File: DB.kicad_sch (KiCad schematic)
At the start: 20 parts

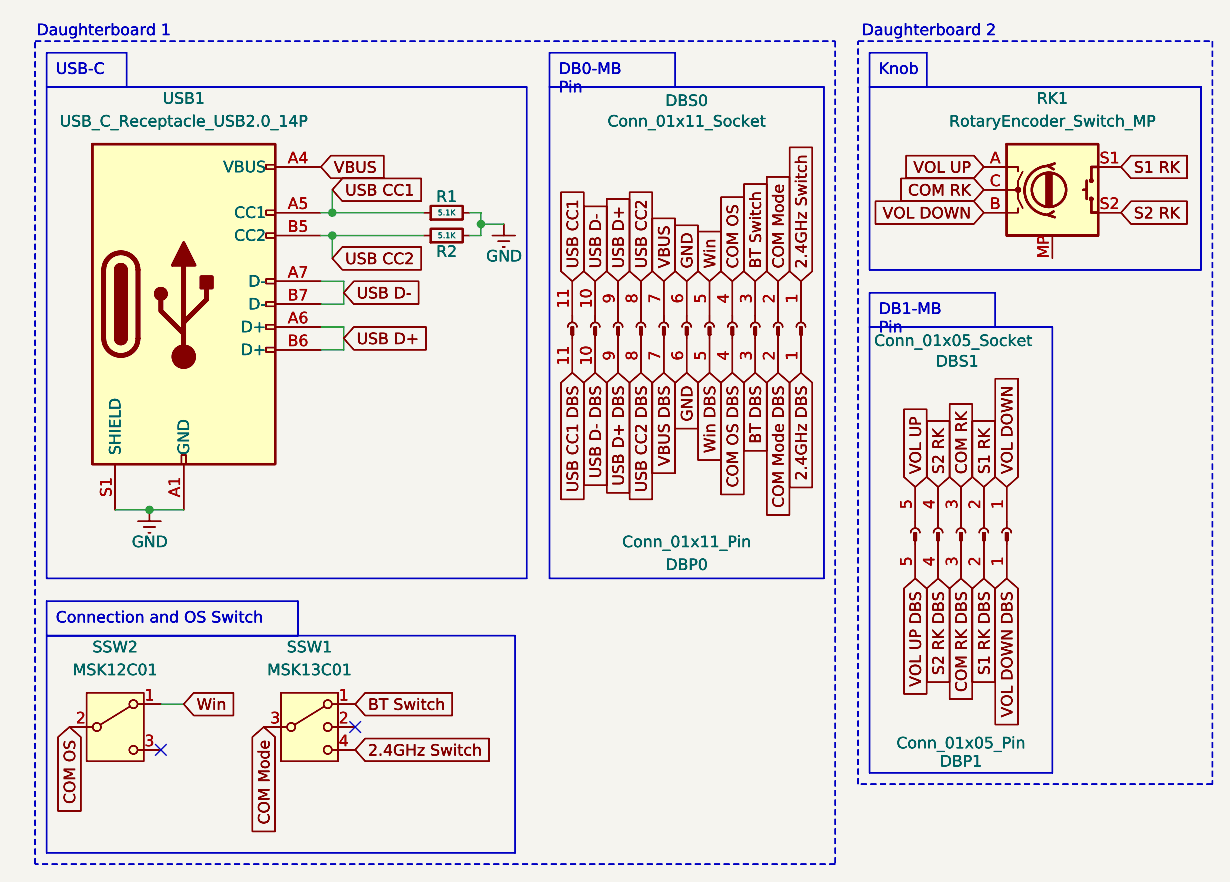
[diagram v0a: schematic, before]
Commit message: Second Commit
new wiring and label
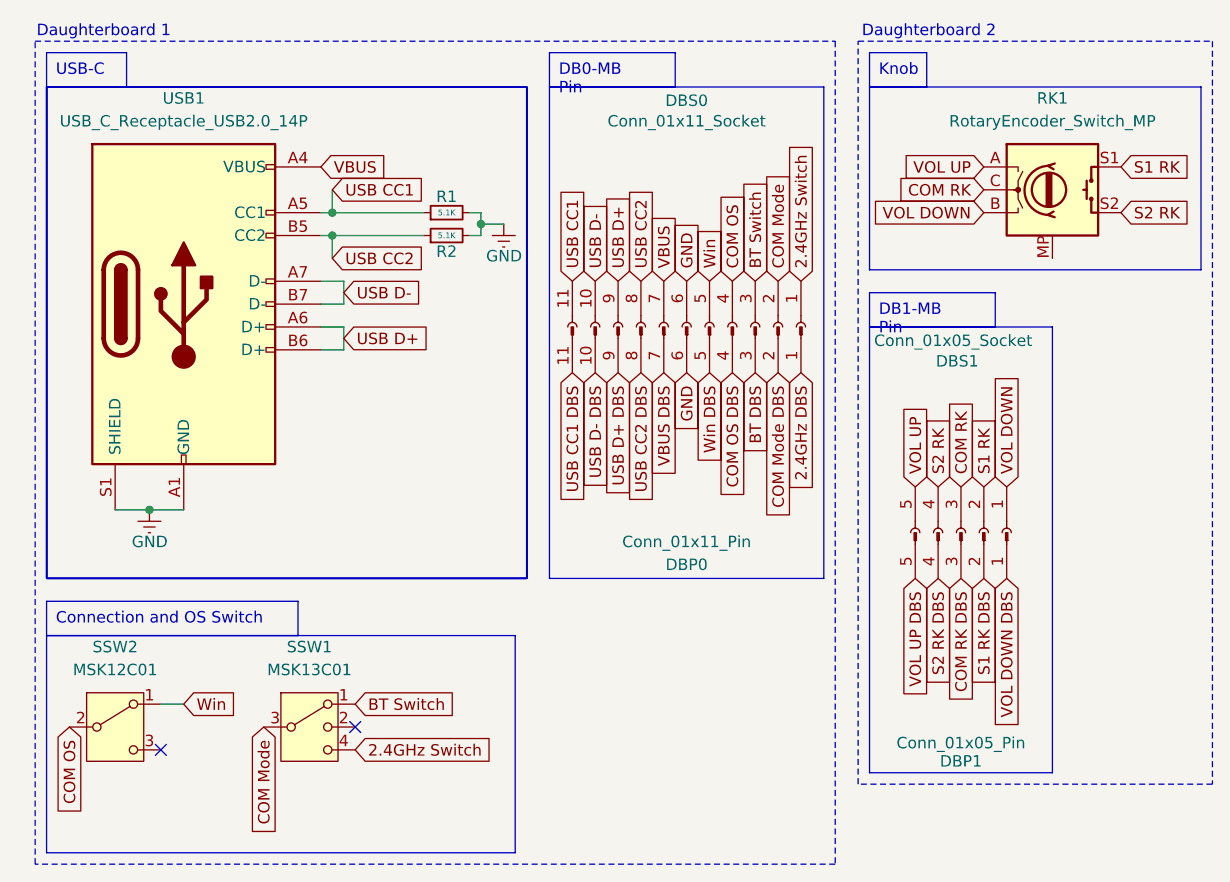
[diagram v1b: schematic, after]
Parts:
- removed DBP0: Conn_01x11_Pin, symbol Connector:Conn_01x11_Pin
- removed DBP1 (x2): Conn_01x05_Pin, symbol Connector:Conn_01x05_Pin
- removed DBS0: Conn_01x11_Socket, Connector_Molex:Molex_PicoBlade_53261-1171_1x11-1MP_P1.25mm_Horizontal, symbol Connector:Conn_01x11_Socket
- removed DBS1: Conn_01x05_Socket, Connector_Molex:Molex_PicoBlade_53261-0571_1x05-1MP_P1.25mm_Horizontal, symbol Connector:Conn_01x05_Socket
- removed R1, R2 (x2): 5.1K, ScottoKeebs_Components:Resistor_0402, symbol Device:R_Small
- removed RK1: RotaryEncoder_Switch_MP, Rotary_Encoder:RotaryEncoder_Alps_EC11E-Switch_Vertical_H20mm, symbol Device:RotaryEncoder_Switch_MP
- removed SSW1 (x2): MSK13C01, Button_Switch_SMD:SW_SP3T_PCM13, symbol Switch:SW_SP3T
- removed SSW2 (x2): MSK12C01, Button_Switch_SMD:SW_SPDT_PCM12, symbol Switch:SW_SPDT
- removed USB1 (x2): USB_C_Receptacle_USB2.0_14P, ScottoKeebs_Components:USB_C_HRO_TYPE-C-31-M-12, symbol Connector:USB_C_Receptacle_USB2.0_14P
- added DBP1: Conn_01x05_Pin, symbol Connector:Conn_01x05_Pin
- added R2: 5.1K, ScottoKeebs_Components:Resistor_0402, symbol Device:R_Small
- added SSW1: MSK13C01, Button_Switch_SMD:SW_SP3T_PCM13, symbol Switch:SW_SP3T
- added SSW2: MSK12C01, Button_Switch_SMD:SW_SPDT_PCM12, symbol Switch:SW_SPDT
- added USB1: USB_C_Receptacle_USB2.0_14P, ScottoKeebs_Components:USB_C_HRO_TYPE-C-31-M-12, symbol Connector:USB_C_Receptacle_USB2.0_14P
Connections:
- net 2.4GHz Switch: now also SSW1.4
- net BT Switch: now also SSW1.1
- net COM Mode: now also SSW1.3
- net COM OS: now also SSW2.2 (B)
- net COM RK DBS: now also DBP1.3 (Pin_3)
- net GND: now also R2.2, USB1.A1 (GND), USB1.A12 (GND), USB1.B1 (GND), USB1.B12 (GND), USB1.S1 (SHIELD)
- net S1 RK DBS: now also DBP1.2 (Pin_2)
- net S2 RK DBS: now also DBP1.4 (Pin_4)
- net USB CC1: now also USB1.A5 (CC1)
- net USB CC2: now also R2.1, USB1.B5 (CC2)
- net USB D+: now also USB1.A6 (D+), USB1.B6 (D+)
- net USB D-: now also USB1.A7 (D-), USB1.B7 (D-)
- net VBUS: now also USB1.A4 (VBUS), USB1.A9 (VBUS), USB1.B4 (VBUS), USB1.B9 (VBUS)
- net VOL DOWN DBS: now also DBP1.1 (Pin_1)
- net VOL UP DBS: now also DBP1.5 (Pin_5)
- net Win: now also SSW2.1 (A)

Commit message: Third Commit
Kinda add some little changes but still confused on how using the nPM1300
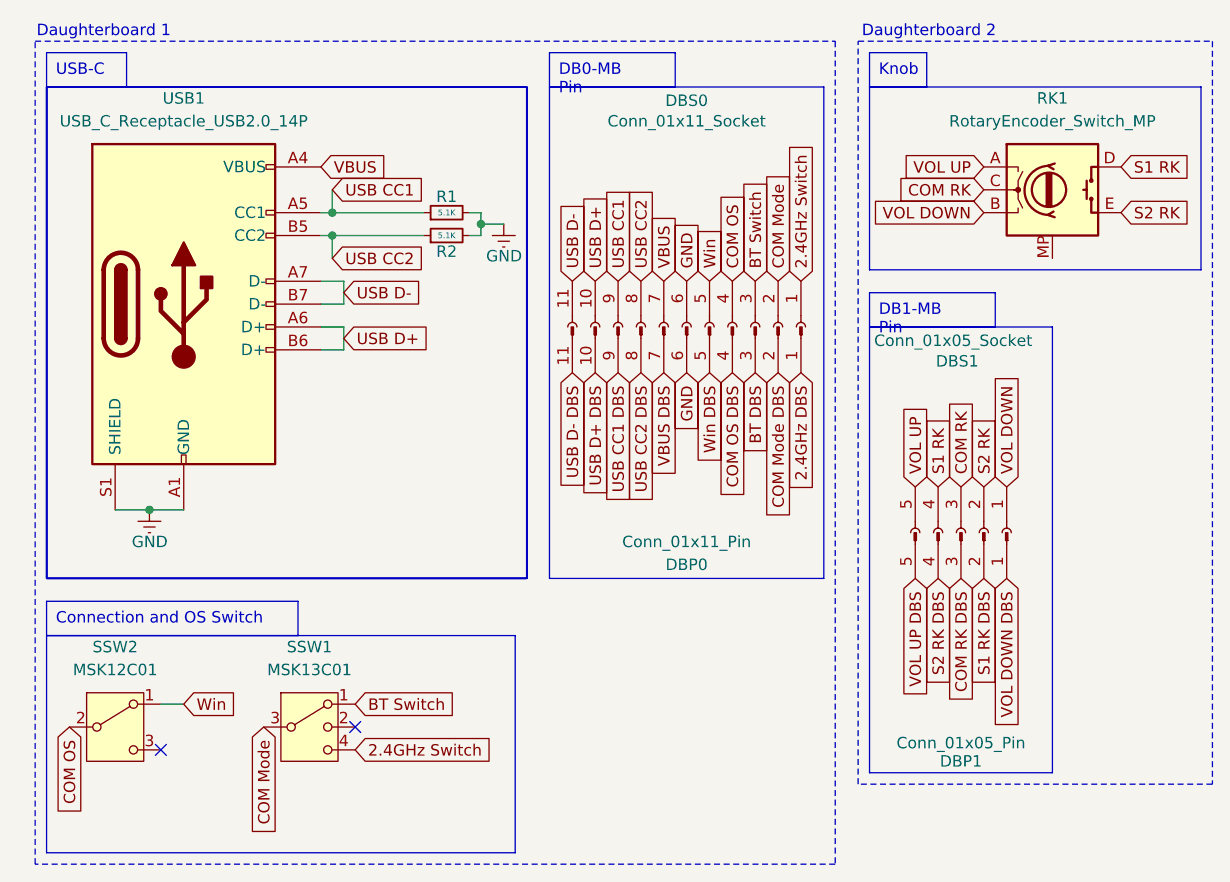
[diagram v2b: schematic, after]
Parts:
- removed RK1: RotaryEncoder_Switch_MP, Rotary_Encoder:RotaryEncoder_Alps_EC11E-Switch_Vertical_H20mm, symbol Device:RotaryEncoder_Switch_MP
- added RK1: RotaryEncoder_Switch_MP, HE_Keyswitch:RotaryEncoder_Bourns_Vertical_PEC11J-9220F-S0015, symbol HE_Keyswitch:RotaryEncoder_Switch_MP
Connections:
- net COM RK: now also RK1.C
- net S1 RK: now also DBS1.4 (Pin_4), RK1.D; no longer DBS1.2 (Pin_2)
- net S2 RK: now also DBS1.2 (Pin_2), RK1.E (S2); no longer DBS1.4 (Pin_4)
- net USB CC1: now also DBS0.9 (Pin_9); no longer DBS0.11 (Pin_11)
- net USB CC1 DBS: now also DBP0.9 (Pin_9); no longer DBP0.11 (Pin_11)
- net USB D+: now also DBS0.10 (Pin_10); no longer DBS0.9 (Pin_9)
- net USB D+ DBS: now also DBP0.10 (Pin_10); no longer DBP0.9 (Pin_9)
- net USB D-: now also DBS0.11 (Pin_11); no longer DBS0.10 (Pin_10)
- net USB D- DBS: now also DBP0.11 (Pin_11); no longer DBP0.10 (Pin_10)
- net VOL DOWN: now also RK1.B
- net VOL UP: now also RK1.A

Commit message: Fourth Commit
changing some name to not get sued :v
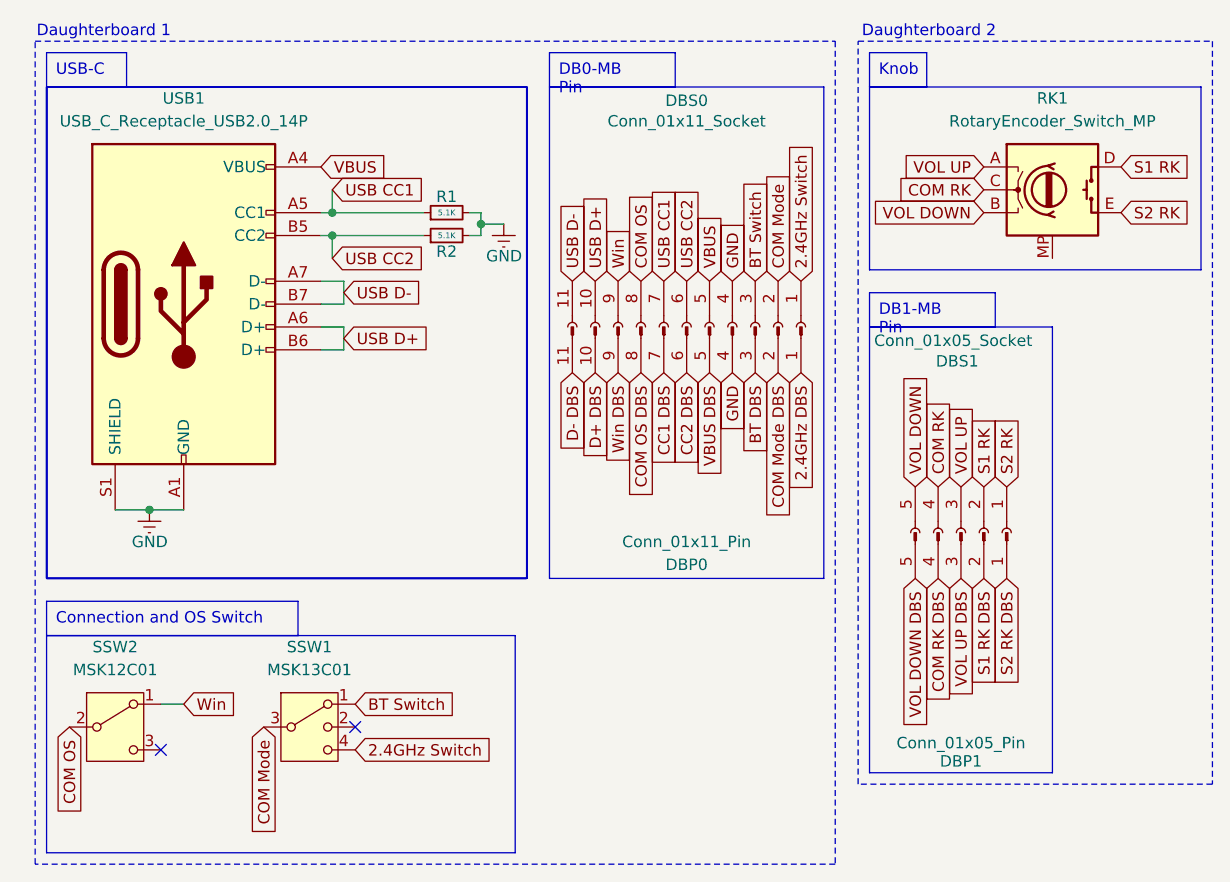
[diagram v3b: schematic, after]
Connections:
- net USB CC1 DBS is gone; now on net Win DBS: DBP0.9 (Pin_9)
- net USB CC2 DBS is gone; now on net COM OS DBS: DBP0.8 (Pin_8)
- net COM OS: now also DBS0.8 (Pin_8); no longer DBS0.4 (Pin_4)
- net COM OS DBS: no longer DBP0.4 (Pin_4)
- net COM RK: now also DBS1.4 (Pin_4); no longer DBS1.3 (Pin_3)
- net COM RK DBS: now also DBP1.4 (Pin_4); no longer DBP1.3 (Pin_3)
- net GND: now also DBP0.4 (Pin_4), DBS0.4 (Pin_4); no longer DBP0.6 (Pin_6), DBS0.6 (Pin_6)
- net S1 RK: now also DBS1.2 (Pin_2); no longer DBS1.4 (Pin_4)
- net S2 RK: now also DBS1.1 (Pin_1); no longer DBS1.2 (Pin_2)
- net S2 RK DBS: now also DBP1.1 (Pin_1); no longer DBP1.4 (Pin_4)
- net USB CC1: now also DBS0.7 (Pin_7); no longer DBS0.9 (Pin_9)
- net USB CC2: now also DBS0.6 (Pin_6); no longer DBS0.8 (Pin_8)
- net VBUS: now also DBS0.5 (Pin_5); no longer DBS0.7 (Pin_7)
- net VBUS DBS: now also DBP0.5 (Pin_5); no longer DBP0.7 (Pin_7)
- net VOL DOWN: now also DBS1.5 (Pin_5); no longer DBS1.1 (Pin_1)
- net VOL DOWN DBS: now also DBP1.5 (Pin_5); no longer DBP1.1 (Pin_1)
- net VOL UP: now also DBS1.3 (Pin_3); no longer DBS1.5 (Pin_5)
- net VOL UP DBS: now also DBP1.3 (Pin_3); no longer DBP1.5 (Pin_5)
- net Win: now also DBS0.9 (Pin_9); no longer DBS0.5 (Pin_5)
- net Win DBS: no longer DBP0.5 (Pin_5)
- net USB D+ DBS renamed D+ DBS
- net USB D- DBS renamed D- DBS
- new net CC1 DBS: DBP0.7 (Pin_7)
- new net CC2 DBS: DBP0.6 (Pin_6)
